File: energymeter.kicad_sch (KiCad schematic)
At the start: 43 parts, among them J1 CT1, J10 CT10, J11 LINE, J12 Conn_02x09_Odd_Even, J13 Conn_02x09_Odd_Even, J2 CT2, J3 CT3, J4 CT4, J5 CT5, J6 CT6, J7 CT7, J8 CT8, J9 CT9, T1 ZMPT107-1, U1 BL-0910, U2 XL1509-3.3, U3 AMS1117-3.3

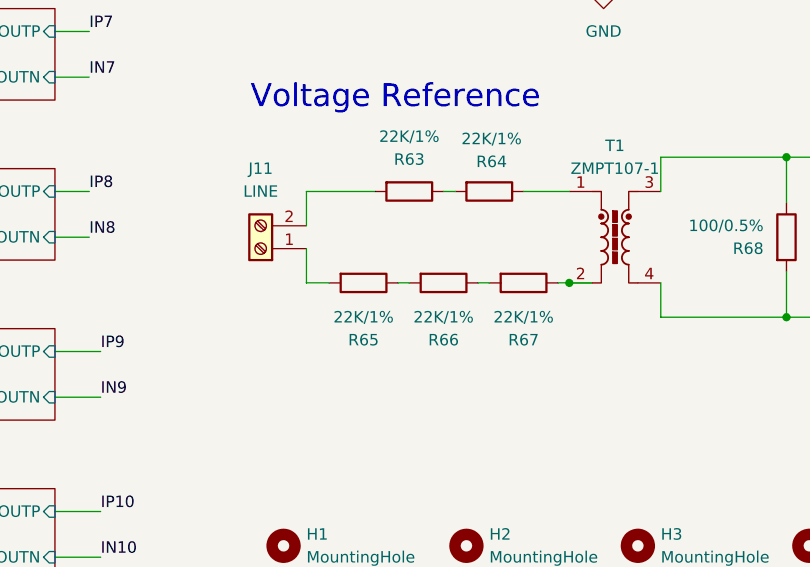
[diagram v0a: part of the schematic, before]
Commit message: Updates
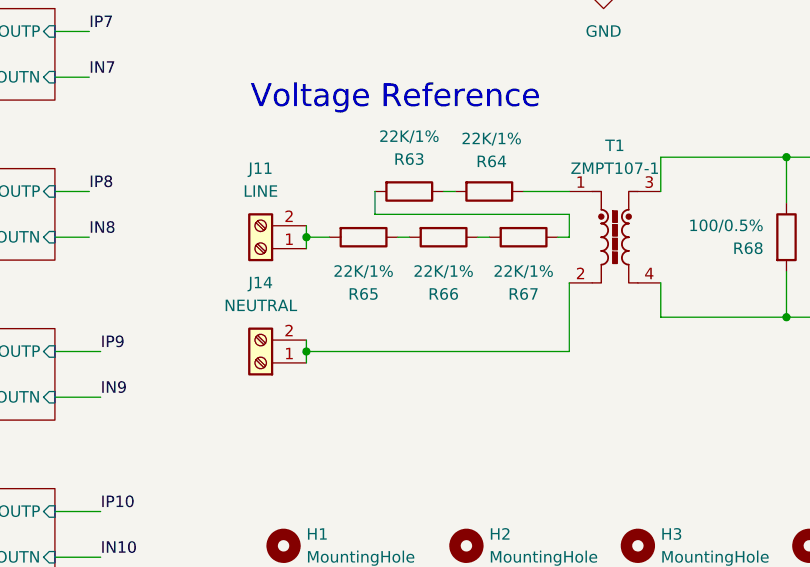
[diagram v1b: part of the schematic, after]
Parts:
- added J14: NEUTRAL, TerminalBlock_Phoenix:TerminalBlock_Phoenix_MKDS-1,5-2_1x02_P5.00mm_Horizontal, symbol Connector:Screw_Terminal_01x02
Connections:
- net at T1.2: now also J14.1 (Pin_1), J14.2 (Pin_2); no longer R67.1
- net at J11.1 (Pin_1), R65.2: now also J11.2 (Pin_2)
- net at R63.2: now also R67.1; no longer J11.2 (Pin_2)
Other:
- moved on the sheet: R65, R66, R67
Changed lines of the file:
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@@
 	)
 	(junction
-		(at 116.84 158.75)
+		(at 87.63 166.37)
 		(diameter 0)
 		(color 0 0 0 0)
@@
 	)
 	(junction
+		(at 87.63 153.67)
+		(diameter 0)
+		(color 0 0 0 0)
+	)
+	(junction
 		(at 162.56 144.78)
 		(diameter 0)
@@
 	(wire
 		(pts
-			(xy 97.79 158.75) (xy 99.06 158.75)
-		)
-		(stroke
-			(width 0)
-			(type default)
-		)
-	)
-	(wire
-		(pts
-			(xy 87.63 158.75) (xy 90.17 158.75)
+			(xy 97.79 153.67) (xy 99.06 153.67)
 		)
 		(stroke
@@
 	(wire
 		(pts
-			(xy 116.84 158.75) (xy 115.57 158.75)
+			(xy 116.84 166.37) (xy 87.63 166.37)
 		)
 		(stroke
@@
 	(wire
 		(pts
+			(xy 87.63 166.37) (xy 87.63 167.64)
+		)
+		(stroke
+			(width 0)
+			(type default)
+		)
+	)
+	(wire
+		(pts
+			(xy 115.57 153.67) (xy 116.84 153.67)
+		)
+		(stroke
+			(width 0)
+			(type default)
+		)
+	)
+	(wire
+		(pts
 			(xy 127 144.78) (xy 140.97 144.78)
 		)
@@
 	(wire
 		(pts
+			(xy 87.63 165.1) (xy 87.63 166.37)
+		)
+		(stroke
+			(width 0)
+			(type default)
+		)
+	)
+	(wire
+		(pts
 			(xy 105.41 38.1) (xy 105.41 41.91)
 		)
@@
 	(wire
 		(pts
+			(xy 87.63 152.4) (xy 87.63 153.67)
+		)
+		(stroke
+			(width 0)
+			(type default)
+		)
+	)
+	(wire
+		(pts
 			(xy 102.87 88.9) (xy 110.49 88.9)
 		)
@@
 	(wire
 		(pts
+			(xy 95.25 151.13) (xy 116.84 151.13)
+		)
+		(stroke
+			(width 0)
+			(type default)
+		)
+	)
+	(wire
+		(pts
 			(xy 217.17 144.78) (xy 217.17 146.05)
 		)
@@
 	(wire
 		(pts
-			(xy 106.68 158.75) (xy 107.95 158.75)
+			(xy 106.68 153.67) (xy 107.95 153.67)
 		)
 		(stroke
@@
 	(wire
 		(pts
+			(xy 116.84 151.13) (xy 116.84 153.67)
+		)
+		(stroke
+			(width 0)
+			(type default)
+		)
+	)
+	(wire
+		(pts
 			(xy 59.69 118.11) (xy 63.5 118.11)
 		)
@@
 	(wire
 		(pts
+			(xy 116.84 158.75) (xy 116.84 166.37)
+		)
+		(stroke
+			(width 0)
+			(type default)
+		)
+	)
+	(wire
+		(pts
 			(xy 27.94 29.21) (xy 27.94 27.94)
 		)
@@
 	(wire
 		(pts
-			(xy 119.38 158.75) (xy 116.84 158.75)
+			(xy 162.56 144.78) (xy 152.4 144.78)
 		)
 		(stroke
@@
 	(wire
 		(pts
-			(xy 162.56 144.78) (xy 152.4 144.78)
+			(xy 90.17 153.67) (xy 87.63 153.67)
 		)
 		(stroke
@@
 	(wire
 		(pts
+			(xy 87.63 153.67) (xy 87.63 154.94)
+		)
+		(stroke
+			(width 0)
+			(type default)
+		)
+	)
+	(wire
+		(pts
 			(xy 140.97 144.78) (xy 140.97 149.86)
 		)
@@
 	(wire
 		(pts
-			(xy 87.63 158.75) (xy 87.63 154.94)
-		)
-		(stroke
-			(width 0)
-			(type default)
-		)
-	)
-	(wire
-		(pts
 			(xy 218.44 95.25) (xy 218.44 97.79)
 		)
@@
 	(wire
 		(pts
-			(xy 87.63 148.59) (xy 87.63 152.4)
-		)
-		(stroke
-			(width 0)
-			(type default)
-		)
-	)
-	(wire
-		(pts
 			(xy 143.51 104.14) (xy 143.51 110.49)
 		)
@@
 	(wire
 		(pts
-			(xy 95.25 148.59) (xy 87.63 148.59)
-		)
-		(stroke
-			(width 0)
-			(type default)
-		)
-	)
-	(wire
-		(pts
 			(xy 218.44 57.15) (xy 220.98 57.15)
 		)
@@
 	(wire
 		(pts
+			(xy 95.25 148.59) (xy 95.25 151.13)
+		)
+		(stroke
+			(width 0)
+			(type default)
+		)
+	)
+	(wire
+		(pts
 			(xy 218.44 41.91) (xy 220.98 41.91)
 		)
@@
 	)
 	(symbol
+		(lib_id "Connector:Screw_Terminal_01x02")
+		(at 82.55 167.64 180)
+		(unit 1)
+		(exclude_from_sim no)
+		(in_bom yes)
+		(on_board yes)
+		(dnp no)
+		(fields_autoplaced yes)
+		(property "Reference" "J14"
+			(at 82.55 158.75 0)
+			(effects
+				(font
+					(size 1.27 1.27)
+				)
+			)
+		)
+		(property "Value" "NEUTRAL"
+			(at 82.55 161.29 0)
+			(effects
+				(font
+					(size 1.27 1.27)
+				)
+			)
+		)
+		(property "Footprint" "TerminalBlock_Phoenix:TerminalBlock_Phoenix_MKDS-1,5-2_1x02_P5.00mm_Horizontal"
+			(at 82.55 167.64 0)
+			(effects
+				(font
+					(size 1.27 1.27)
+				)
+				(hide yes)
+			)
+		)
+		(property "Datasheet" "~"
+			(at 82.55 167.64 0)
+			(effects
+				(font
+					(size 1.27 1.27)
+				)
+				(hide yes)
+			)
+		)
+		(property "Description" "Generic screw terminal, single row, 01x02, script generated (kicad-library-utils/schlib/autogen/connector/)"
+			(at 82.55 167.64 0)
+			(effects
+				(font
+					(size 1.27 1.27)
+				)
+				(hide yes)
+			)
+		)
+		(pin "2"
+		)
+		(pin "1"
+		)
+		(instances
+			(project "energymeter"
+				(path "/d5c3d4dc-7952-499c-ae9a-397827d02ad2"
+					(reference "J14")
+					(unit 1)
+				)
+			)
+		)
+	)
+	(symbol
 		(lib_id "power:+3.3V")
 		(at 259.08 128.27 0)
@@
 	(symbol
 		(lib_id "Device:R")
-		(at 111.76 158.75 270)
+		(at 111.76 153.67 270)
 		(unit 1)
 		(exclude_from_sim no)
@@
 		(fields_autoplaced yes)
 		(property "Reference" "R67"
-			(at 111.76 165.1 90)
+			(at 111.76 160.02 90)
 			(effects
 				(font
@@
 		)
 		(property "Value" "22K/1%"
-			(at 111.76 162.56 90)
+			(at 111.76 157.48 90)
 			(effects
 				(font
@@
 		)
 		(property "Footprint" "Resistor_SMD:R_0603_1608Metric"
-			(at 111.76 156.972 90)
+			(at 111.76 151.892 90)
 			(effects
 				(font
@@
 		)
 		(property "Datasheet" "~"
-			(at 111.76 158.75 0)
+			(at 111.76 153.67 0)
 			(effects
 				(font
@@
 		)
 		(property "Description" "Resistor"
-			(at 111.76 158.75 0)
+			(at 111.76 153.67 0)
 			(effects
 				(font
@@
 	(symbol
 		(lib_id "Device:R")
-		(at 102.87 158.75 270)
+		(at 102.87 153.67 270)
 		(unit 1)
 		(exclude_from_sim no)
@@
 		(fields_autoplaced yes)
 		(property "Reference" "R66"
-			(at 102.87 165.1 90)
+			(at 102.87 160.02 90)
 			(effects
 				(font
@@
 		)
 		(property "Value" "22K/1%"
-			(at 102.87 162.56 90)
+			(at 102.87 157.48 90)
 			(effects
 				(font
@@
 		)
 		(property "Footprint" "Resistor_SMD:R_0603_1608Metric"
-			(at 102.87 156.972 90)
+			(at 102.87 151.892 90)
 			(effects
 				(font
@@
 		)
 		(property "Datasheet" "~"
-			(at 102.87 158.75 0)
+			(at 102.87 153.67 0)
 			(effects
 				(font
@@
 		)
 		(property "Description" "Resistor"
-			(at 102.87 158.75 0)
+			(at 102.87 153.67 0)
 			(effects
 				(font
@@
 	(symbol
 		(lib_id "Device:R")
-		(at 93.98 158.75 270)
+		(at 93.98 153.67 270)
 		(unit 1)
 		(exclude_from_sim no)
@@
 		(fields_autoplaced yes)
 		(property "Reference" "R65"
-			(at 93.98 165.1 90)
+			(at 93.98 160.02 90)
 			(effects
 				(font
@@
 		)
 		(property "Value" "22K/1%"
-			(at 93.98 162.56 90)
+			(at 93.98 157.48 90)
 			(effects
 				(font
@@
 		)
 		(property "Footprint" "Resistor_SMD:R_0603_1608Metric"
-			(at 93.98 156.972 90)
+			(at 93.98 151.892 90)
 			(effects
 				(font
@@
 		)
 		(property "Datasheet" "~"
-			(at 93.98 158.75 0)
+			(at 93.98 153.67 0)
 			(effects
 				(font
@@
 		)
 		(property "Description" "Resistor"
-			(at 93.98 158.75 0)
+			(at 93.98 153.67 0)
 			(effects
 				(font
